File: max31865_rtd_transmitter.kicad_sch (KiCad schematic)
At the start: 37 parts, among them J4 SM03B-SRSS-TB, SW2 SW_Push, U7 NCP1117-3.3_SOT223, U8 RP2350_60QFN, U9 W25Q32JVZPIQ, Y1 ABM8-272-T3

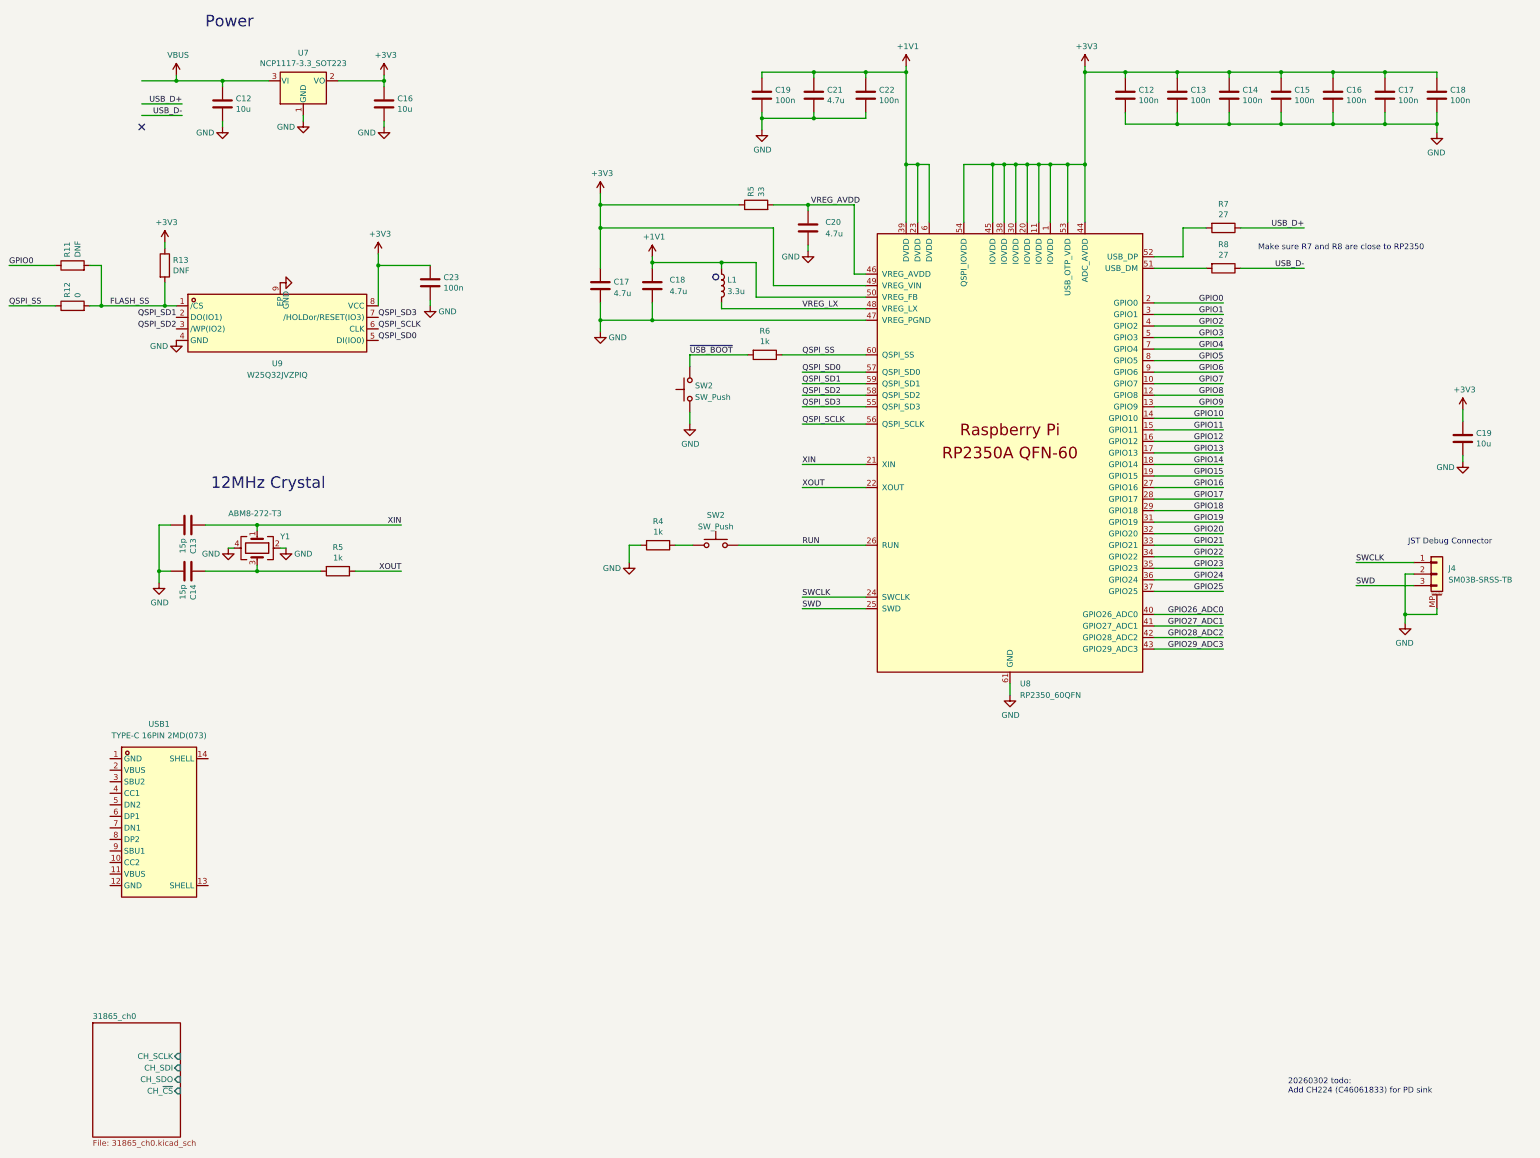
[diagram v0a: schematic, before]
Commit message: complete schematic layout
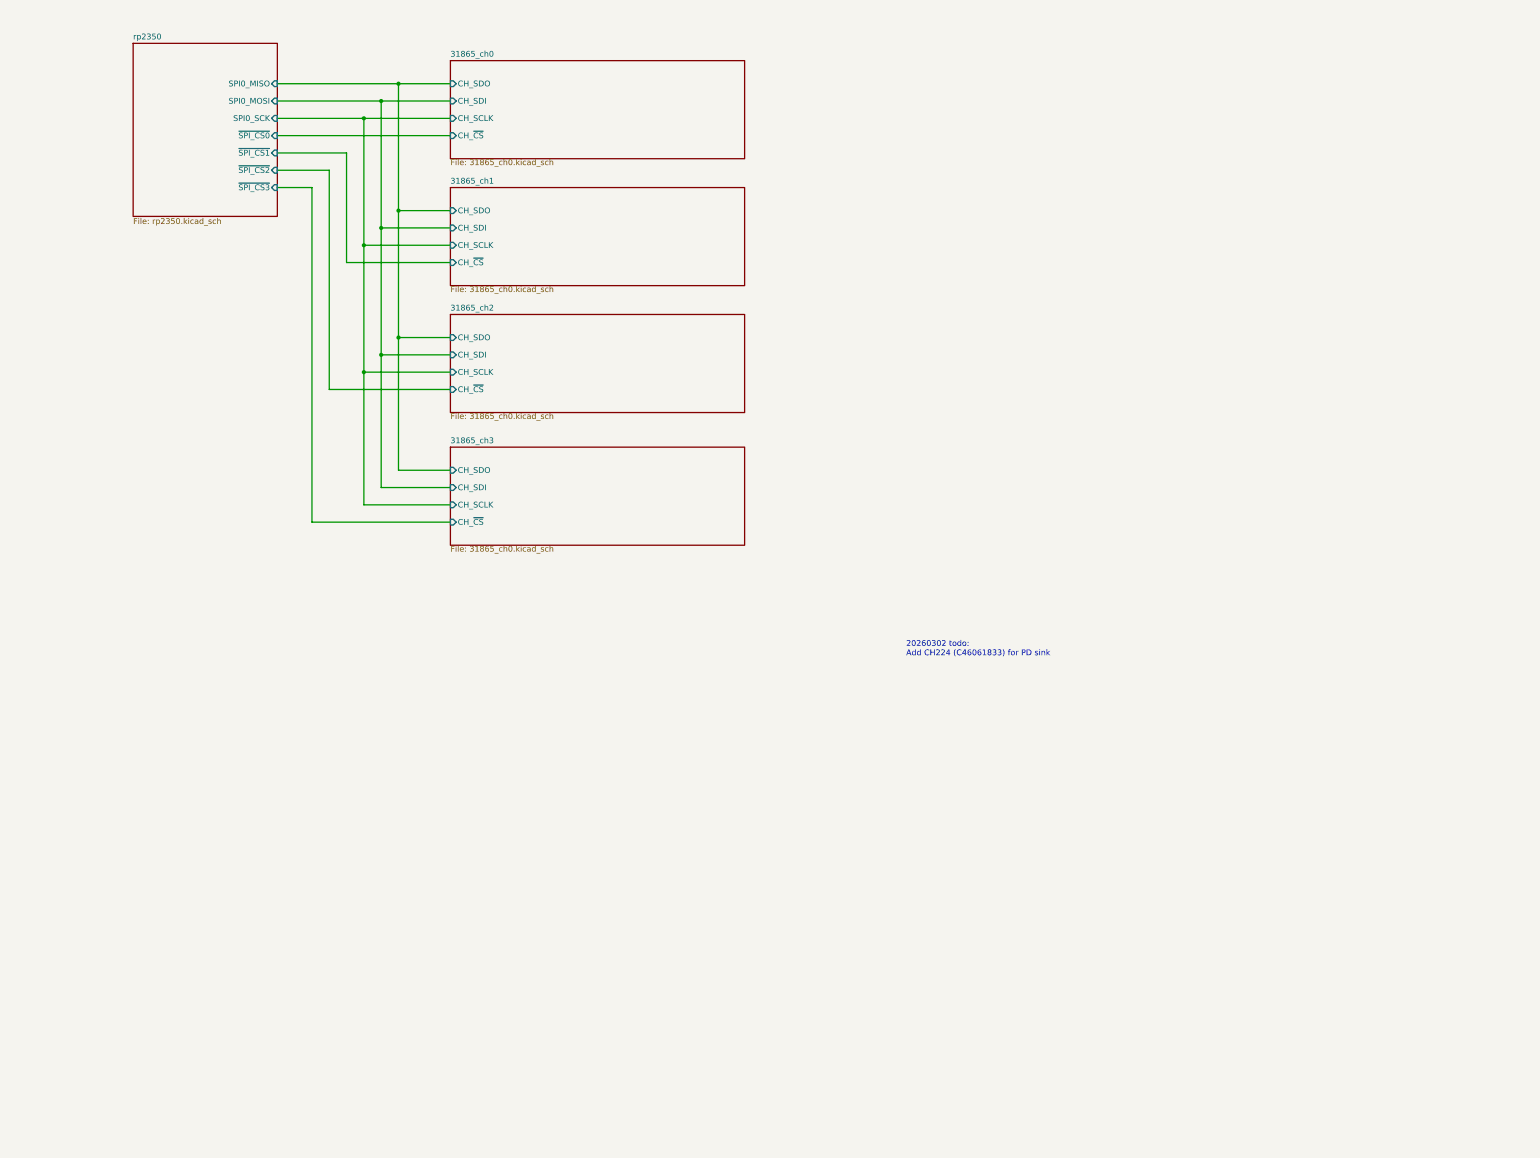
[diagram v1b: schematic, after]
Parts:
- removed C12, C13, C14, C15, C16, C17, C18, C19, C22, C23: 100n, Capacitor_SMD:C_0402_1005Metric, symbol Device:C
- removed C12, C16, C19: 10u, Capacitor_SMD:C_0805_2012Metric, symbol Device:C
- removed C13, C14: 15p, Capacitor_SMD:C_0402_1005Metric, symbol Device:C
- removed C17, C18: 4.7u, RP2350_60QFN_minimal:C_0402_1005Metric_small_pads, symbol Device:C
- removed C20, C21: 4.7u, Capacitor_SMD:C_0402_1005Metric, symbol Device:C
- removed J4: SM03B-SRSS-TB, Connector_JST:JST_SH_SM03B-SRSS-TB_1x03-1MP_P1.00mm_Horizontal, symbol Connector_Generic_MountingPin:Conn_01x03_MountingPin
- removed L1: 3.3u, RP2350_60QFN_minimal:L_pol_2016, symbol Device:L
- removed R11, R13: DNF, Resistor_SMD:R_0402_1005Metric, symbol Device:R
- removed R12: 0, Resistor_SMD:R_0402_1005Metric, symbol Device:R
- removed R4, R5, R6: 1k, Resistor_SMD:R_0402_1005Metric, symbol Device:R
- removed R5: 33, Resistor_SMD:R_0402_1005Metric, symbol Device:R
- removed R7, R8: 27, Resistor_SMD:R_0402_1005Metric, symbol Device:R
- removed SW2 (x2): SW_Push, Button_Switch_SMD:SW_Push_1P1T_NO_Vertical_Wuerth_434133025816, symbol Switch:SW_Push
- removed U7: NCP1117-3.3_SOT223, Package_TO_SOT_SMD:SOT-223-3_TabPin2, symbol Regulator_Linear:NCP1117-3.3_SOT223
- removed U8: RP2350_60QFN, RP2350_60QFN_minimal:RP2350-QFN-60-1EP_7x7_P0.4mm_EP3.4x3.4mm_ThermalVias, symbol MCU_RaspberryPi_RP2350:RP2350_60QFN
- removed U9: W25Q32JVZPIQ, rtd-transmitter-library:WSON-8_L6.0-W5.0-P1.27-BL-EP, symbol rtd-transmitter-library:W25Q32JVZPIQ
- removed USB1: TYPE-C 16PIN 2MD(073), rtd-transmitter-library:USB-C-SMD_TYPE-C-6PIN-2MD-073, symbol rtd-transmitter-library:TYPE-C16PIN2MD(073)
- removed Y1: ABM8-272-T3, Crystal:Crystal_SMD_3225-4Pin_3.2x2.5mm, symbol Device:Crystal_GND24
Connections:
- no-connect marks 1 -> 0
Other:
- added sheet 31865_ch1 (31865_ch0.kicad_sch)
- added sheet 31865_ch2 (31865_ch0.kicad_sch)
- added sheet 31865_ch3 (31865_ch0.kicad_sch)
- added sheet rp2350 (rp2350.kicad_sch)
- note removed: "12MHz Crystal"
- note removed: "JST Debug Connector"
- note removed: "Make sure R7 and R8 are close to RP2350"
- note removed: "Power"
